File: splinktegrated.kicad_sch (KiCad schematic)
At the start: 62 parts, among them J1 USB_C_Receptacle_USB2.0, J10 NA_Ribbon, J13 Conn_01x01_Socket, J14 Cirque, J15 Conn_01x01_Socket, J16 Conn_01x01_Socket, J17 Conn_01x01_Socket, J18 USB_C_Receptacle_USB2.0, J5 Conn_01x02, J6 Cirque, J7 NA_trackball, J8 NA_Ribbon, J9 NA_RGB, Q4 AO3401A, Q5 AO3401A, SW1 NA_SW_SPST, SW2 NA_SW_SPST, U1 RP2040, U2 USBLC6-2P6, U3 XC6210B332MR-G, U4 USBLC6-2P6, U5 W25Q128JVS, Y1 Crystal_GND24

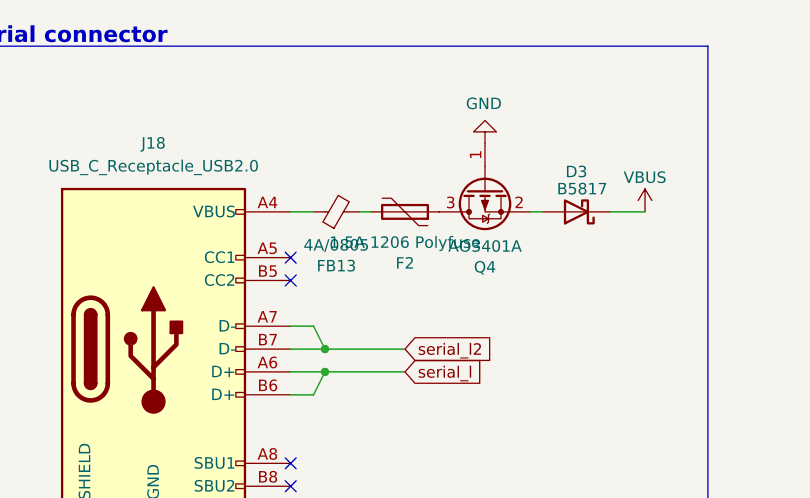
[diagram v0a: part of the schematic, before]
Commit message: BOM work
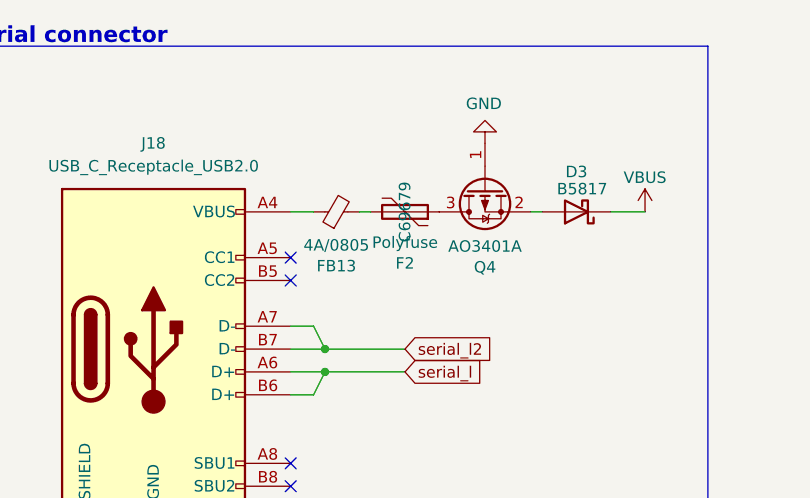
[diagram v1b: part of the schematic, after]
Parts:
- F2: value 1.5A 1206 Polyfuse -> Polyfuse; footprint reversible-kicad-footprints:Fuse_1206_3216Metric -> Fuse:Fuse_0603_1608Metric; LCSC (none) -> C69679
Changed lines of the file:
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@@
 			)
 		)
-		(property "Value" "1.5A 1206 Polyfuse"
+		(property "Value" "Polyfuse"
 			(at -140.97 30.0736 90)
 			(effects
@@
 			)
 		)
-		(property "Footprint" "reversible-kicad-footprints:Fuse_1206_3216Metric"
+		(property "Footprint" "Fuse:Fuse_0603_1608Metric"
 			(at -146.05 25.4 0)
 			(effects
@@
 			(at -140.97 26.67 0)
 			(effects
+				(font
+					(size 1.27 1.27)
+				)
+			)
+		)
+		(property "LCSC" "C69679"
+			(at -140.97 26.67 0)
+			(effects
